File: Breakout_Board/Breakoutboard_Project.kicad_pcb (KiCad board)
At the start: 2 copper layers, 37 parts, among them U1 ADXL380-2BCCZ-RL7, U2 STM32F411, U3 ICM-40609-D, U4 MMC5983MA, U5 BMP581

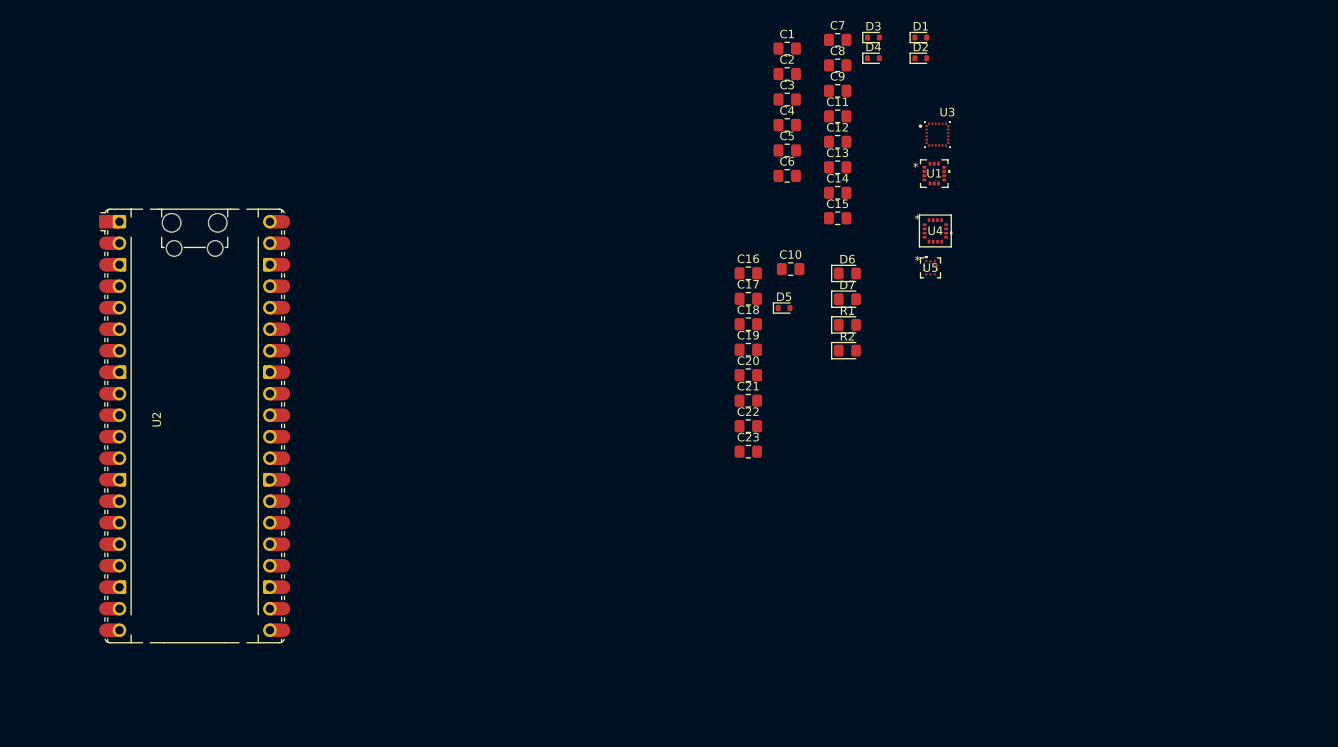
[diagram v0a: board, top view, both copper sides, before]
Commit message: some layout
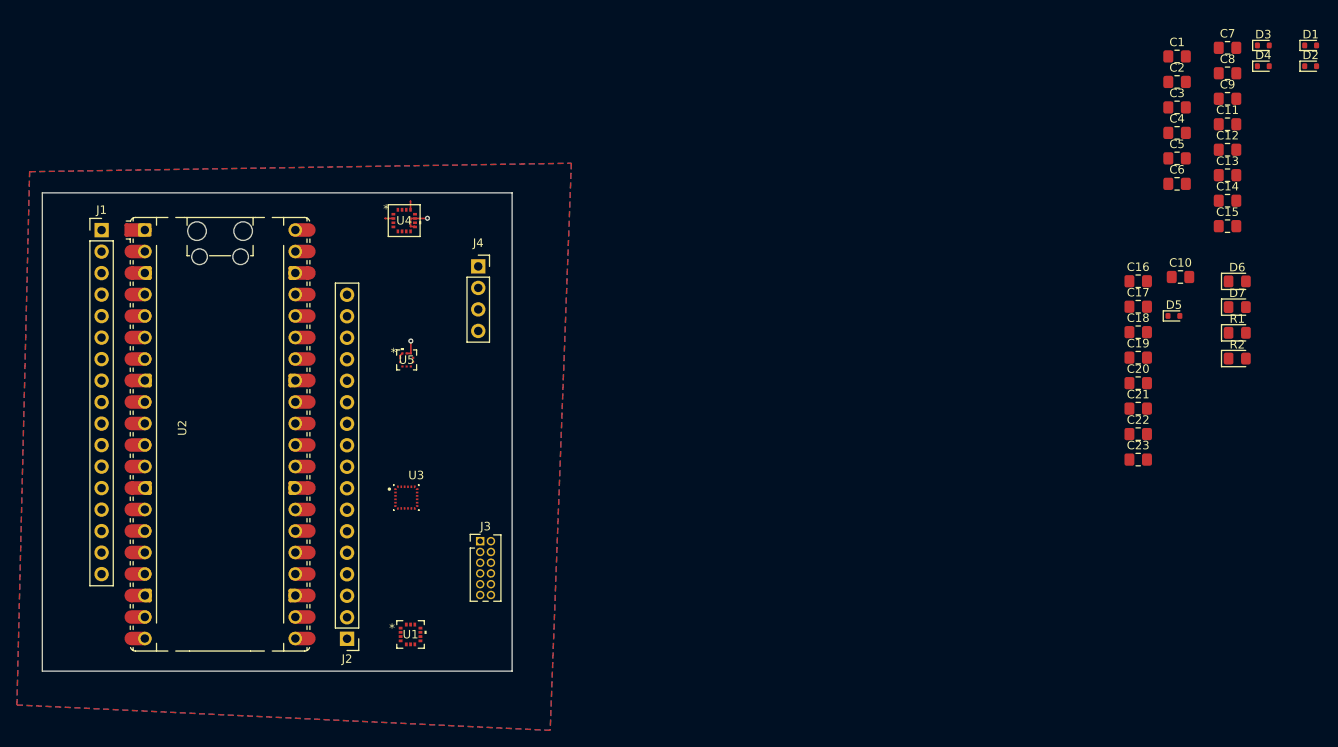
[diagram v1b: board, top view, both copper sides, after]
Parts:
- added J1: Conn_01x17, Connector_PinHeader_2.54mm:PinHeader_1x17_P2.54mm_Vertical, F.Cu at (28.0, 36.9)
- added J2: Conn_01x17, Connector_PinHeader_2.54mm:PinHeader_1x17_P2.54mm_Vertical, F.Cu at (57.0, 85.2)
- added J3: Conn_02x06_Top_Bottom, Connector_PinHeader_1.27mm:PinHeader_2x06_P1.27mm_Vertical, F.Cu at (72.7, 73.7)
- added J4: Conn_01x04, Connector_PinSocket_2.54mm:PinSocket_1x04_P2.54mm_Vertical, F.Cu at (72.5, 41.2)
- moved U1 82.4 mm to (64.5, 84.7)
- moved U3 76.0 mm to (64.0, 68.5)
- moved U5 62.8 mm to (64.0, 52.2)
- moved U4 62.8 mm to (63.8, 35.8)
- moved C1 46.1 mm to (155.1, 16.4)
- moved C10 46.1 mm to (155.5, 42.4)
- moved C11 46.1 mm to (161.0, 24.4)
- moved C12 46.1 mm to (161.0, 27.4)
- moved C13 46.1 mm to (161.0, 30.4)
- moved C14 46.1 mm to (161.0, 33.4)
- moved C15 46.1 mm to (161.0, 36.4)
- moved C16 46.1 mm to (150.5, 42.9)
- moved C17 46.1 mm to (150.5, 46.0)
- moved C18 46.1 mm to (150.5, 49.0)
- moved C19 46.1 mm to (150.5, 52.0)
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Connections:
- U2 pad 1: unconnected-(U2-B12-Pad1) -> /B12
- U2 pad 13: unconnected-(U2-B5-Pad13) -> /B5
- U2 pad 14: unconnected-(U2-15-Pad14) -> /B6
- U2 pad 15: unconnected-(U2-B7-Pad15) -> /B7
- U2 pad 16: unconnected-(U2-B8-Pad16) -> /B8
- U2 pad 17: unconnected-(U2-B9-Pad17) -> /B9
- U2 pad 21: unconnected-(U2-VB-Pad21) -> /VB
- U2 pad 22: unconnected-(U2-C13-Pad22) -> /C13
- U2 pad 23: unconnected-(U2-C14-Pad23) -> /C14
- U2 pad 24: unconnected-(U2-C15-Pad24) -> /C15
- U2 pad 25: unconnected-(U2-R-Pad25) -> /R
- U2 pad 26: unconnected-(U2-A0-Pad26) -> /A0
- U2 pad 34: unconnected-(U2-B0-Pad34) -> /B0
- U2 pad 35: unconnected-(U2-B1-Pad35) -> /B1
- U2 pad 36: unconnected-(U2-B2-Pad36) -> /B2
- U2 pad 37: unconnected-(U2-B10-Pad37) -> /B10
- U2 pad 4: unconnected-(U2-B15-Pad4) -> /B15
- U2 pad 5: unconnected-(U2-A8-Pad5) -> /A8
- U2 pad 6: unconnected-(U2-A9-Pad6) -> /A9
- U2 pad 7: unconnected-(U2-A10-Pad7) -> /A10
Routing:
- net GND: track 0.00 -> 5.46 mm, vias 0 -> 2
- net +3.3V: track 0.00 -> 2.62 mm
- added copper zone on F.Cu, net +3.3V
- added copper zone on B.Cu, net GND
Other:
- board outline added: 55.5 x 56.5 mm

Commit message: helo
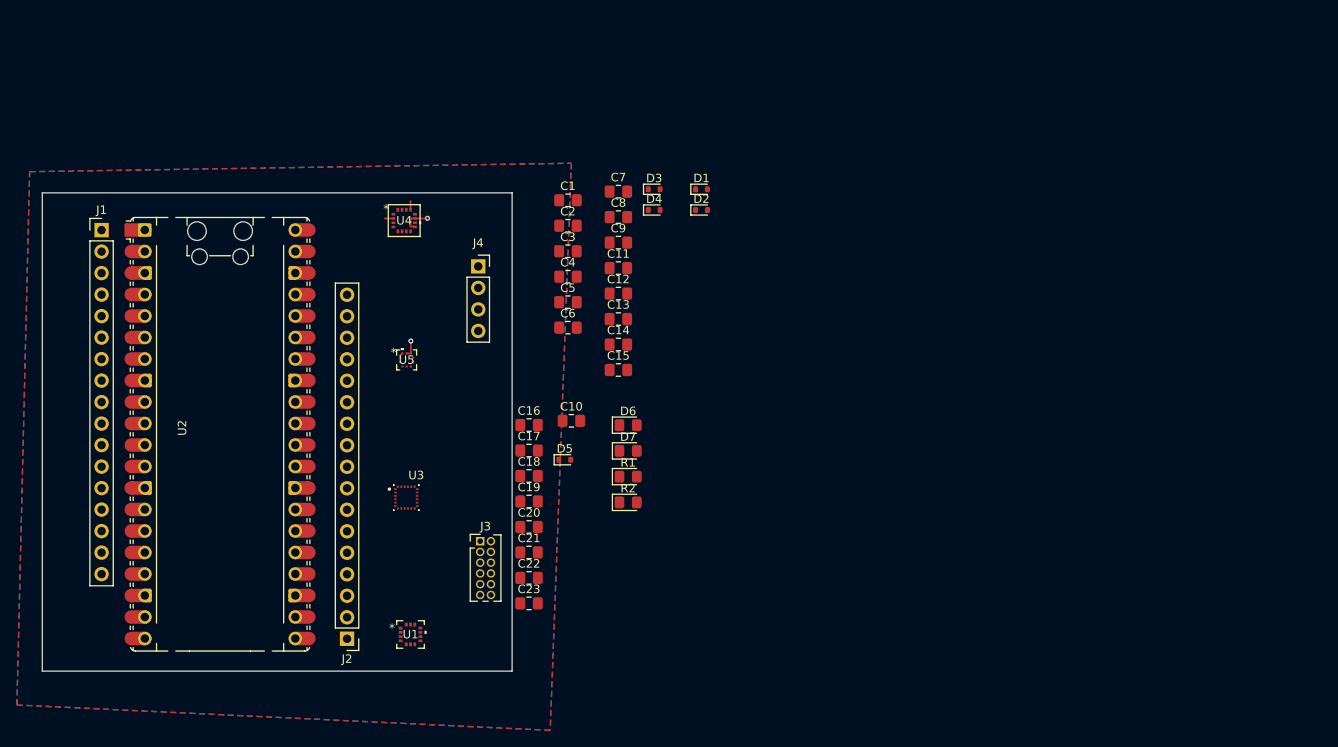
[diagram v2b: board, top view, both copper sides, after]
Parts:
- moved C1 73.9 mm to (83.1, 33.4)
- moved C10 73.9 mm to (83.5, 59.4)
- moved C11 73.9 mm to (89.1, 41.4)
- moved C12 73.9 mm to (89.1, 44.4)
- moved C13 73.9 mm to (89.1, 47.4)
- moved C14 73.9 mm to (89.1, 50.4)
- moved C15 73.9 mm to (89.1, 53.4)
- moved C16 73.9 mm to (78.5, 59.9)
- moved C17 73.9 mm to (78.5, 62.9)
- moved C18 73.9 mm to (78.5, 66.0)
- moved C19 73.9 mm to (78.5, 69.0)
- moved C2 73.9 mm to (83.1, 36.4)
- moved C20 73.9 mm to (78.5, 72.0)
- moved C21 73.9 mm to (78.5, 75.0)
- moved C22 73.9 mm to (78.5, 78.0)
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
